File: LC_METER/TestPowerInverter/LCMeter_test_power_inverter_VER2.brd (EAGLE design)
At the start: 60 x 28 mm, 64 parts, among them IC1 MC34063, IC10 MC34063, T1 H772, T2 H772, X1 VCC_IN, X2 GND, X3 +5V_STAB, X4 +8.5V_STAB, X5 -8.5V, X6 GND

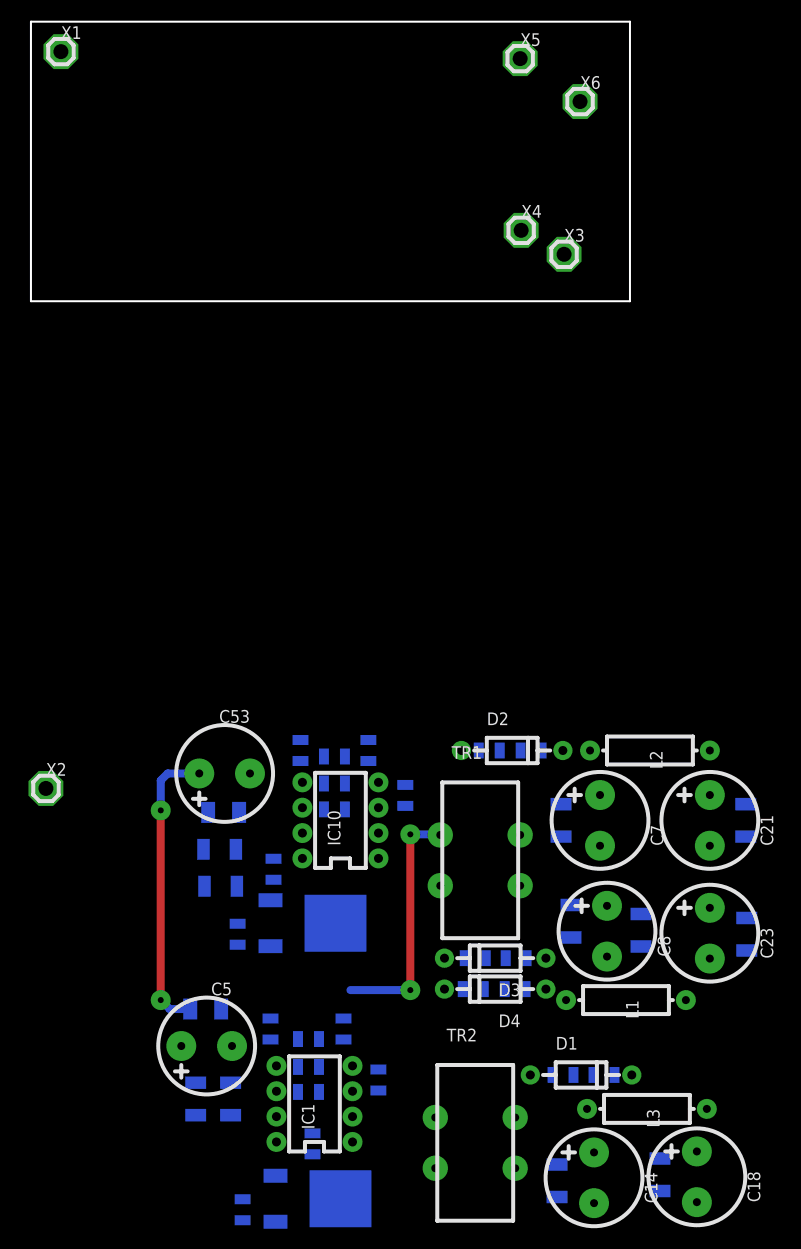
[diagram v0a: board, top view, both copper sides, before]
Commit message: PowerInverter_V2
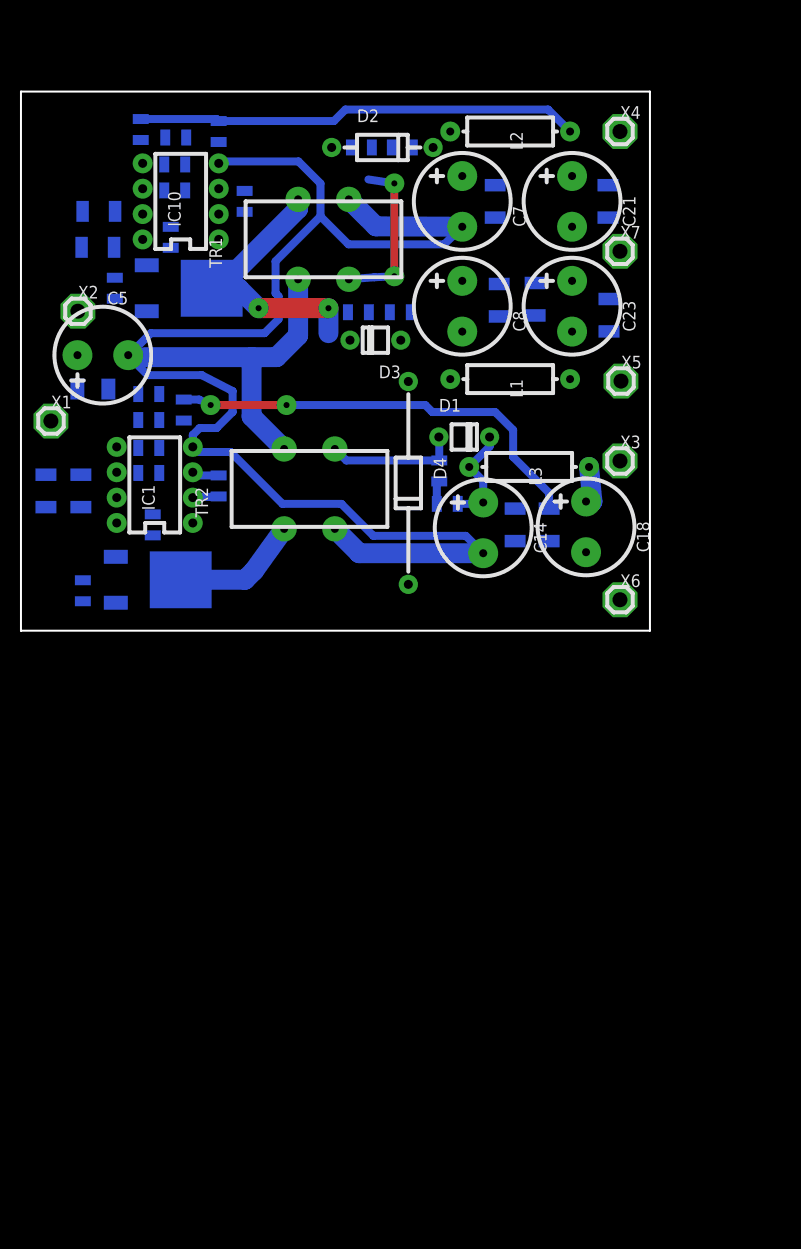
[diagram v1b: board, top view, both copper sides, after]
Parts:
- removed C4: 1n0, __MyCommonLib1:RSMD_0805
- removed C53: 1000uFx16V, __MyCommonLib1:CE_10MM
- removed C54: 0.47uFx16V, __MyCommonLib1:RSMD_1206
- removed R14: 10R, __MyCommonLib1:RSMD_0805
- added X7: GND, __MyCommonLib1:PIN1X1_3.5MM_PWR
- D1, D3: device __MyCommonLib1:DO-41_10MM -> __MyCommonLib1:DO-41_5MM
- D4: device __MyCommonLib1:DO-41_10MM -> __MyCommonLib1:DO-41_20MM
- moved C5 70.0 mm to (8.20, 27.6)
- moved TR2 67.6 mm to (28.9, 14.2), turned to 90 degrees
- moved C18 66.0 mm to (56.6, 10.4)
- moved C14 66.0 mm to (46.3, 10.3)
- moved C19 66.0 mm to (52.9, 10.6)
- moved R2 65.9 mm to (9.40, 34.3)
- moved C13 65.8 mm to (49.5, 10.6)
- moved R4 65.7 mm to (33.8, 31.9)
- moved C1 65.7 mm to (38.0, 31.9)
- moved L3 65.4 mm to (50.9, 16.4)
- moved R83 65.2 mm to (7.70, 38.4)
- moved R3 65.0 mm to (7.80, 42.0)
- moved D1 65.0 mm to (44.4, 19.4)
- moved T1 64.8 mm to (19.1, 34.3)
- moved R9 64.8 mm to (12.8, 23.7), turned to 180 degrees
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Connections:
- removed net N$13: C4.PAD_1, R14.PAD_0
- net GND: now also TR2.W1_START, TR2.W2_END, X7.1; no longer C53.MINUS, C54.PAD_0, TR2.W1_END, TR2.W2_START
- net N$12: now also TR2.W1_END; no longer R14.PAD_1, TR2.W2_END
- net N$14: now also TR2.W2_START; no longer TR2.W1_START
- net N$17: no longer C4.PAD_0
- net N$4: now also TR1.W1_START; no longer TR1.W2_END
- net N$8: now also TR1.W2_END; no longer TR1.W1_START
- net VCC_IN: no longer C53.PLUS, C54.PAD_1
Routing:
- net GND: track 24.6 -> 176.1 mm, vias 2 -> 0
- net +5V_STABILIZED: track 0.00 -> 47.7 mm, vias 0 -> 2
- net +8.5V_STABILIZED: track 0.00 -> 44.5 mm
- net VCC_IN: track 29.4 -> 0.00 mm, vias 2 -> 0
- net N$4: track 0.28 -> 26.5 mm, vias 0 -> 2
- net N$8: track 0.00 -> 16.5 mm, vias 0 -> 2
- net N$14: track 0.00 -> 13.3 mm
- net N$12: track 0.00 -> 12.9 mm
- net N$18: track 0.00 -> 10.6 mm
- net N$7: track 0.00 -> 2.72 mm
- net N$15: track 0.00 -> 2.35 mm
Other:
- board size 60 x 28 mm -> 63 x 54 mm
